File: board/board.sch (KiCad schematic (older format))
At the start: 46 parts, among them Q1 FDV305N, Q2 FDV305N, Q3 FDV305N, U1 STM32F405RGTx, U2 TPS542941, Y1 16MHz

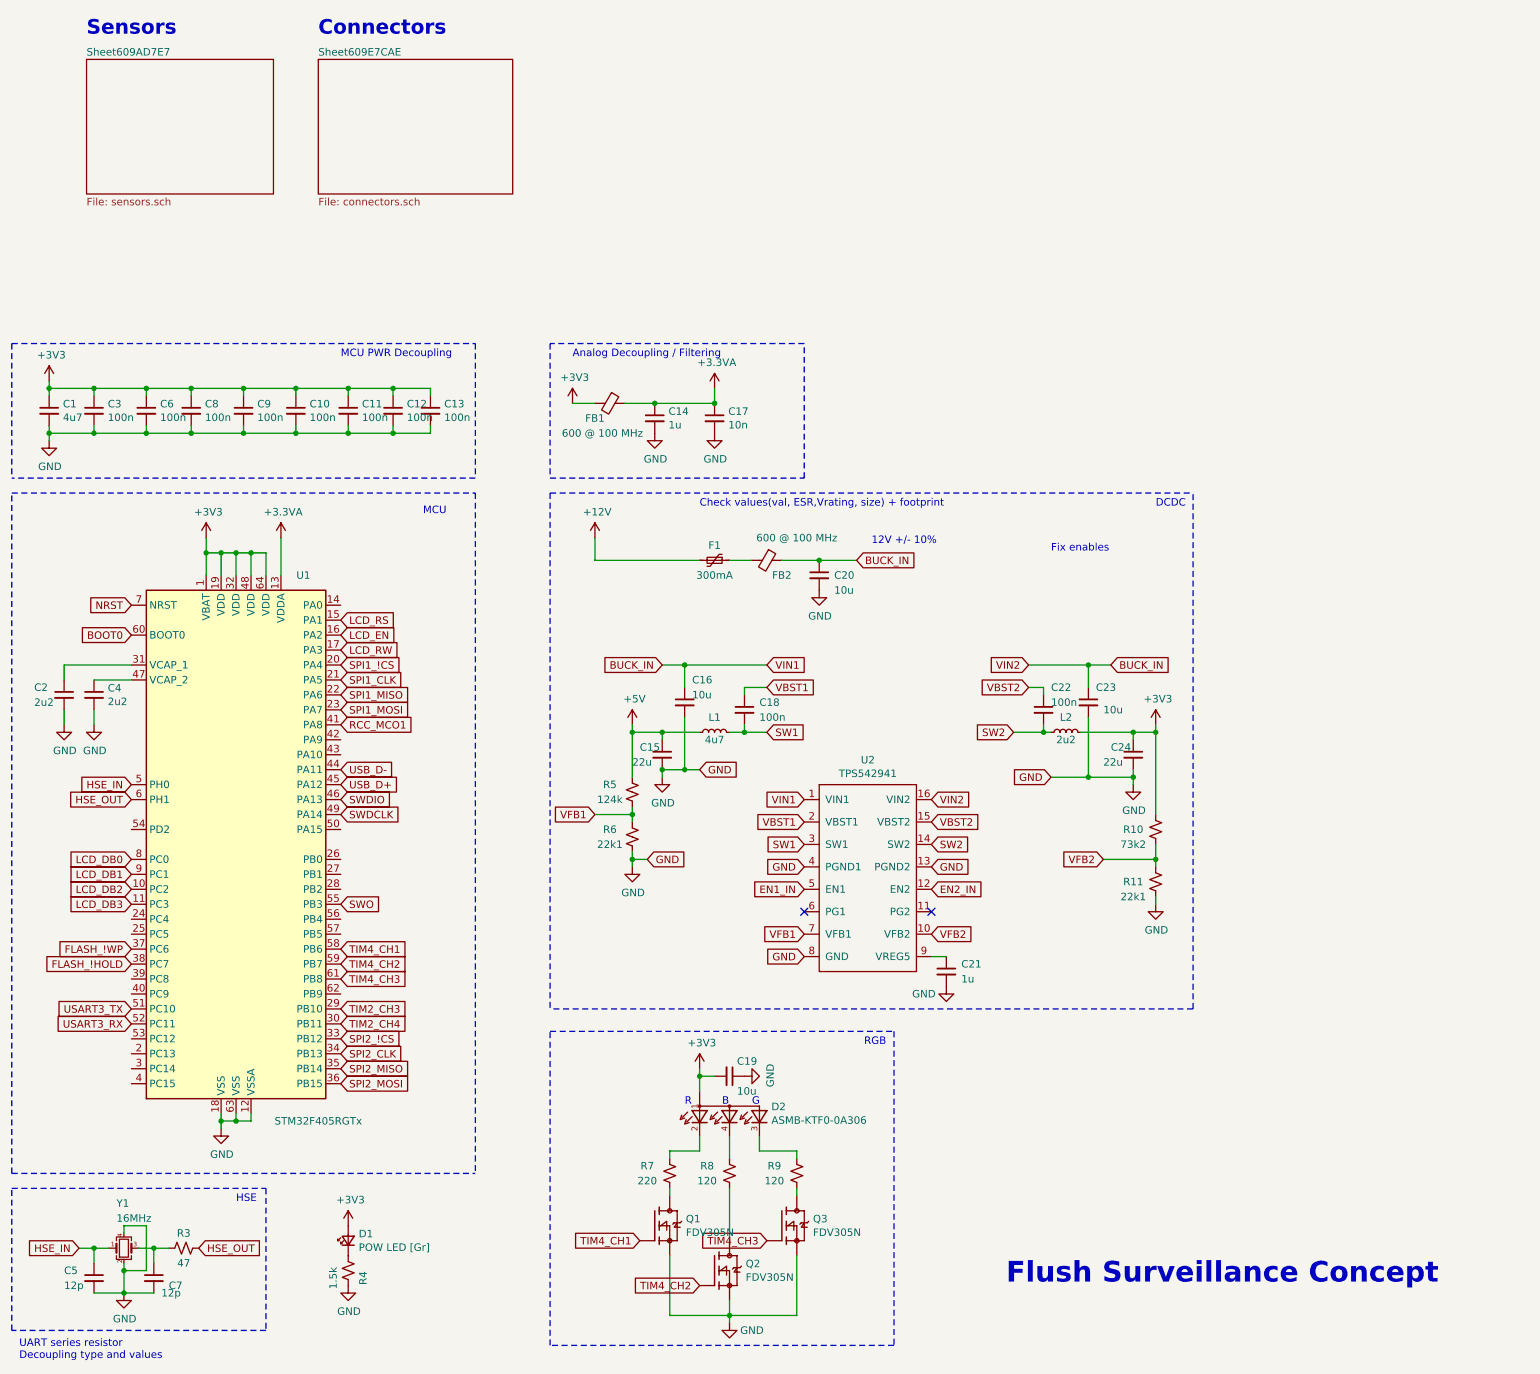
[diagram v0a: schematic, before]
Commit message: Push
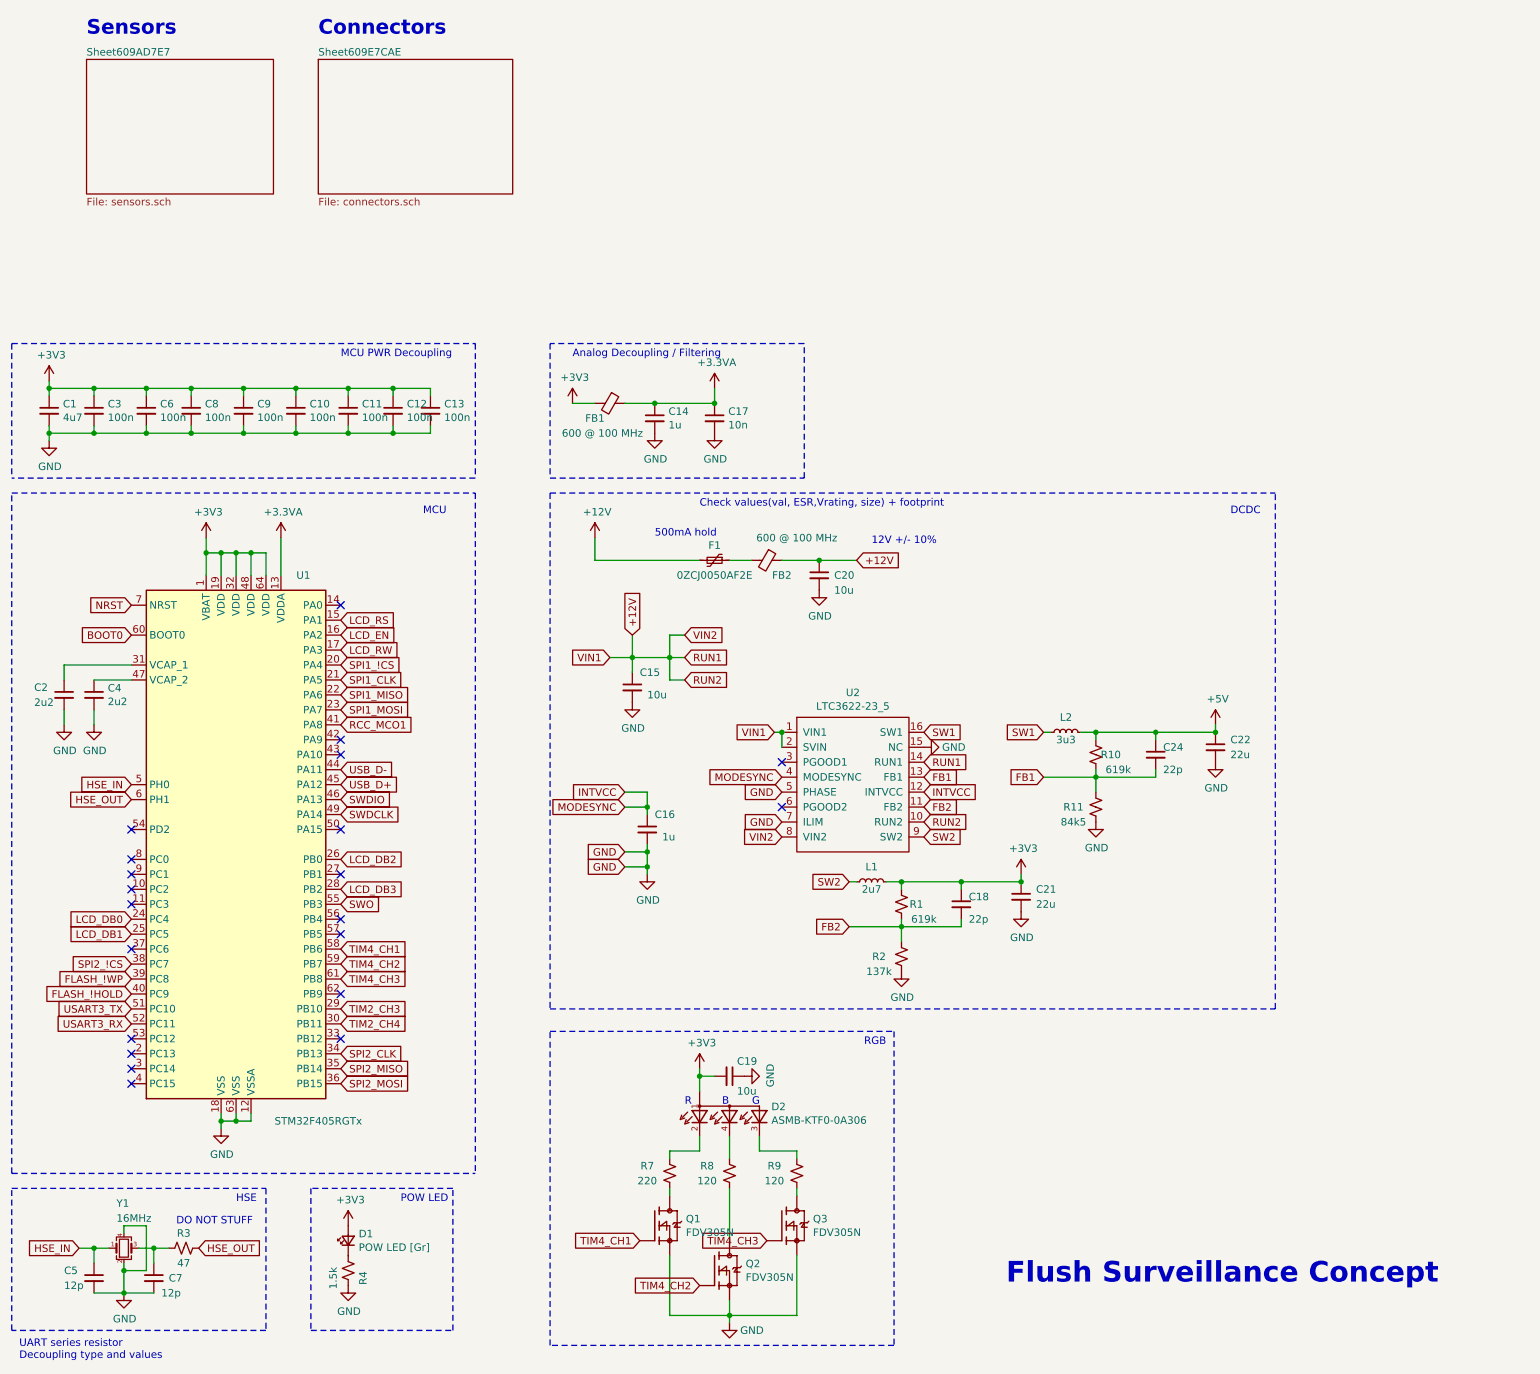
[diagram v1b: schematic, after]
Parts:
- removed C23: 10u, Capacitor_SMD:C_0603_1608Metric, symbol Device:C_Small
- removed R5: 124k, Resistor_SMD:R_0603_1608Metric, symbol Device:R_Small_US
- removed R6: 22k1, Resistor_SMD:R_0603_1608Metric, symbol Device:R_Small_US
- removed U2: TPS542941, Package_SO:HTSSOP-16-1EP_4.4x5mm_P0.65mm_EP3.4x5mm_Mask2.46x2.31mm_ThermalVias, symbol board-rescue:TPS542941
- added R1: 619k, Resistor_SMD:R_0402_1005Metric, symbol Device:R_Small_US
- added R2: 137k, Resistor_SMD:R_0402_1005Metric, symbol Device:R_Small_US
- added U2: LTC3622-23_5, Package_SO:MSOP-16-1EP_3x4mm_P0.5mm_EP1.65x2.85mm_ThermalVias, symbol board-rescue:LTC3622-23_5
- C15: value 22u -> 10u
- C16: value 10u -> 1u; footprint Capacitor_SMD:C_0603_1608Metric -> Capacitor_SMD:C_0402_1005Metric
- C18: value 100n -> 22p; footprint Capacitor_SMD:C_0603_1608Metric -> Capacitor_SMD:C_0402_1005Metric
- C21: value 1u -> 22u; footprint Capacitor_SMD:C_0603_1608Metric -> Capacitor_SMD:C_0402_1005Metric
- C22: value 100n -> 22u; footprint Capacitor_SMD:C_0603_1608Metric -> Capacitor_SMD:C_0402_1005Metric
- C24: value 22u -> 22p; footprint Capacitor_SMD:C_0603_1608Metric -> Capacitor_SMD:C_0402_1005Metric
- C5, C7: LSCS Part # (none) -> C32949
- F1: value 300mA -> 0ZCJ0050AF2E
- L1: value 4u7 -> 2u7
- L2: value 2u2 -> 3u3; LCSC Part # (none) -> C370336
- Q1, Q2, Q3: footprint SOT95P240X111-3N -> FDV305N:SOT95P240X111-3N
- R10: value 73k2 -> 619k; footprint Resistor_SMD:R_0603_1608Metric -> Resistor_SMD:R_0402_1005Metric
- R11: value 22k1 -> 84k5; footprint Resistor_SMD:R_0603_1608Metric -> Resistor_SMD:R_0402_1005Metric
- R3: LCSC Part # (none) -> C478874
- Y1: LCSC Part # (none) -> C13738
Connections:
- net VBST1 is gone; now on net +3V3: C18.1
- net VBST2 is gone; now on net +5V: C22.1
- net +12V: now also C15.1, C20.1, FB2.1, U2.1 (VIN1), U2.10 (RUN2), U2.14 (RUN1), U2.2 (SVIN), U2.8 (VIN2)
- net +3V3: now also C21.1, L1.2, R1.2; no longer C24.1, L2.2, R10.2
- net +5V: now also C24.1, L2.2, R10.2; no longer C15.1, L1.1
- net FLASH_!HOLD: now also U1.40 (PC9); no longer U1.38 (PC7)
- net FLASH_!WP: now also U1.39 (PC8); no longer U1.37 (PC6)
- net GND: now also C22.2, R2.1, U2.15 (NC), U2.5 (PHASE), U2.7 (ILIM); no longer C24.2
- net LCD_DB0: now also U1.24 (PC4); no longer U1.8 (PC0)
- net LCD_DB1: now also U1.25 (PC5); no longer U1.9 (PC1)
- net LCD_DB2: now also U1.26 (PB0); no longer U1.10 (PC2)
- net LCD_DB3: now also U1.28 (PB2); no longer U1.11 (PC3)
- net SPI2_!CS: now also U1.38 (PC7); no longer U1.33 (PB12)
- net SW1: now also L2.1, U2.16 (SW1); no longer C18.2, L1.2
- net SW2: now also L1.1, U2.9 (SW2); no longer C22.2, L2.1
- removed net BUCK_IN: C16.1, C20.1, FB2.1
- net VFB2 renamed FB1
- net FB1: now also C24.2, U2.13 (FB1)
- new net FB2: C18.2, R1.1, R2.2, U2.11 (FB2)
- new net INTVCC: C16.1, U2.12 (INTVCC), U2.4 (MODESYNC)
- no-connect marks 2 -> 21
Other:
- note added: "500mA hold\n"
- note added: "DO NOT STUFF\n"
- note added: "POW LED"
- note removed: "Fix enables\n"
- moved on the sheet: C24, R10, R11
